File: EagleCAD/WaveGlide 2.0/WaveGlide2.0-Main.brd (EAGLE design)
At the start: 100 x 100 mm, 8 parts, among them IC1 TPS77033, K1 AQY21SOP, K2 MS-20-310-HN, U1 ATMEGA328P_TQFP, U2 BMP180, U3 MPXV7002, X1 22-23-2111

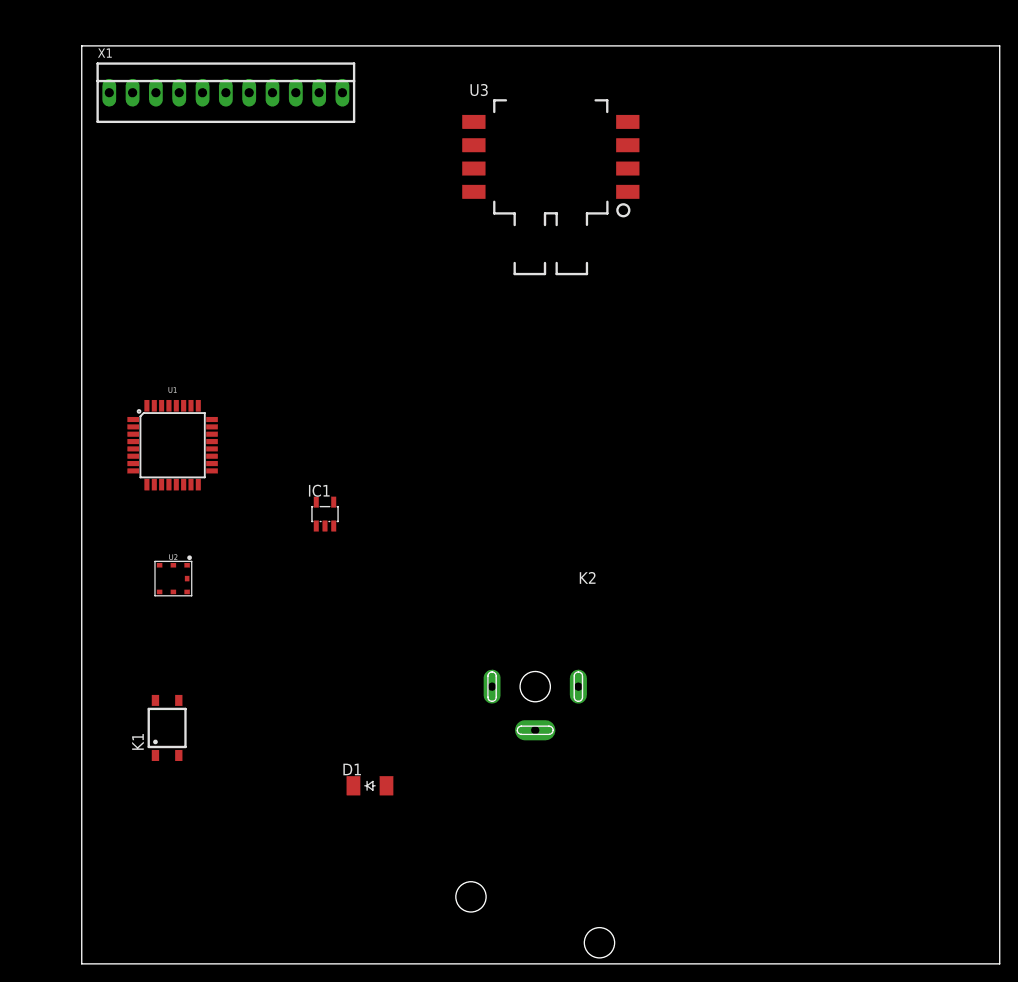
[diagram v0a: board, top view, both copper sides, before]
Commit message: Updated Schematic
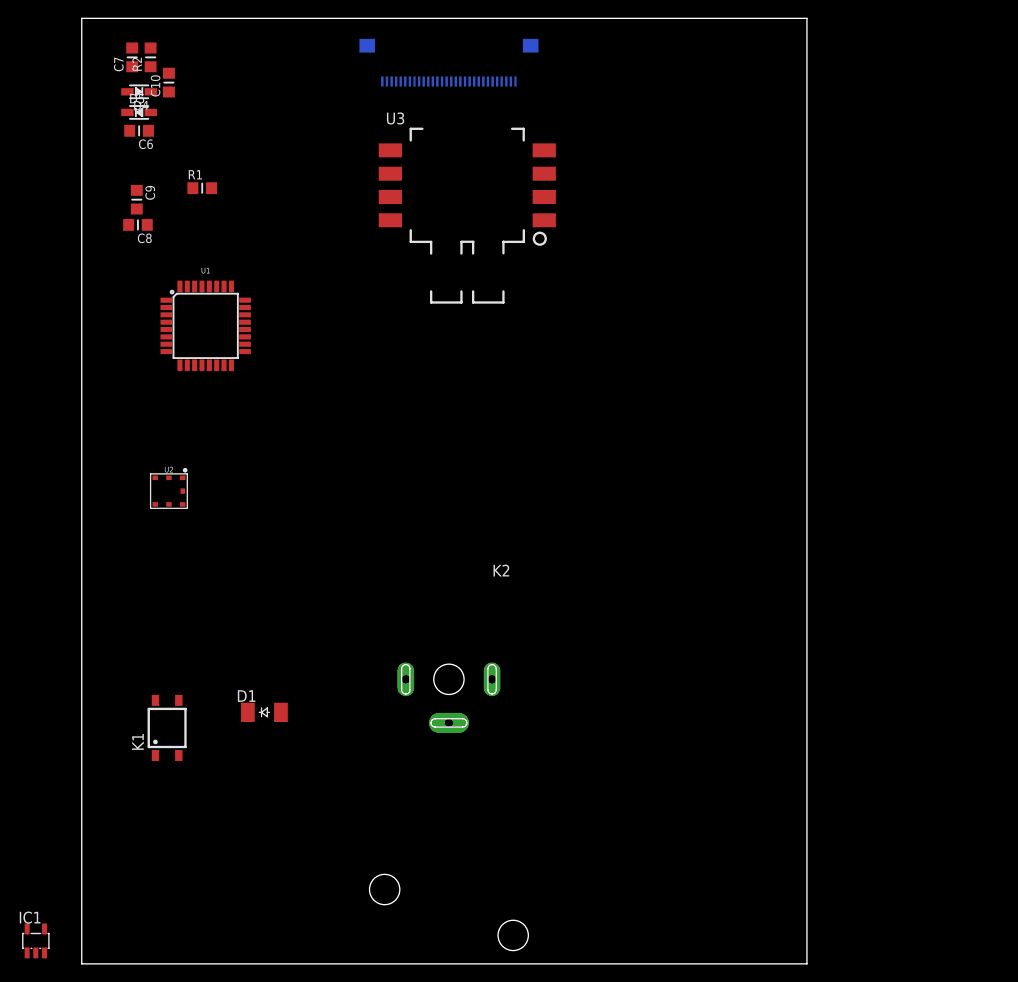
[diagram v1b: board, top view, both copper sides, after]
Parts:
- removed X1: 22-23-2111, con-molex:22-23-2111
- added C10, C6: 10uF/16V, microbuilder:_0805MP
- added C7, C8: 1.0uF, microbuilder:_0805MP
- added C9: 10uF, microbuilder:_0805MP
- added D4, D5: 1N4148, microbuilder:SOD-323
- added R1: 560k, microbuilder:_0805MP
- added R2: 50, microbuilder:_0805MP
- added U5: UG-2828GDEDF11, microbuilder:FPC_XF2M-3015-1A
- IC1: device texas:SOT23-DBV -> CustomParts:SOT23-DBV
- U1: device SparkFun-IC-Microcontroller:TQFP32-08 -> CustomParts:TQFP32-08
- U2: device SparkFun-Sensors:BMP180 -> CustomParts:BMP180
- moved IC1 56.2 mm to (-5.00, 2.50)
- moved D1 14.0 mm to (19.9, 27.4)
- moved U1 13.5 mm to (13.5, 69.5)
- moved U3 9.61 mm to (42.0, 81.0)
- moved U2 9.54 mm to (9.50, 51.5)
- moved K2 9.43 mm to (40.0, 31.0)
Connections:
- new net 13V: C6.1, U5.P$29
- new net 3V3: C7.1, C9.1, U5.P$27, U5.P$4
- new net N$2: D4.A, R2.1
- new net N$3: C10.1, U5.P$28
- new net N$4: U5.P$5
- new net N$5: D4.C, D5.A
- new net N$6: C8.1
- new net N$7: R1.2, U5.P$9
- new net N$8: R2.2, U5.P$26
- new net OLED_BS0: U5.P$14
- new net OLED_CS: U5.P$12
- new net OLED_DC: U5.P$11
- new net OLED_MOSI: U5.P$18
- new net OLED_RES: U5.P$10
- new net OLED_SCK: U5.P$17
- net GND: now also C10.2, C6.2, C7.2, C8.2, C9.2, D5.C, K2.3, R1.1, U5.P$1, U5.P$13, U5.P$3, U5.P$30; no longer K2.P$3
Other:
- board size 100 x 100 mm -> 79 x 103 mm
